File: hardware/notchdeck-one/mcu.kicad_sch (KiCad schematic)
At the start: 10 parts, among them J3 SWD, J4 TC2030_NL, U1 E73-2G4M08S1C

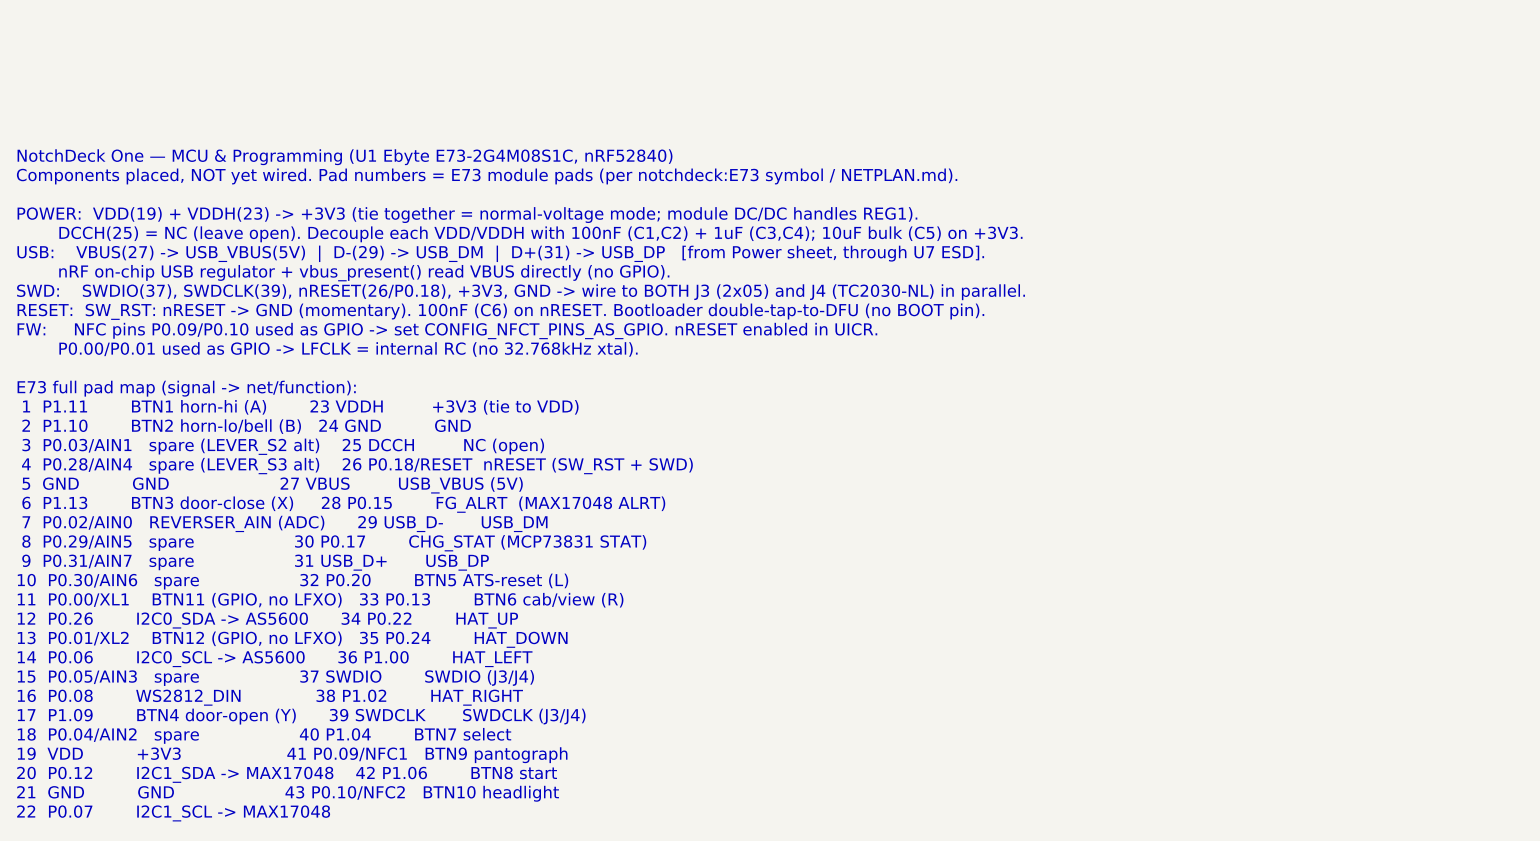
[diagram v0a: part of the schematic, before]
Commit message: Add schematic wiring notes support
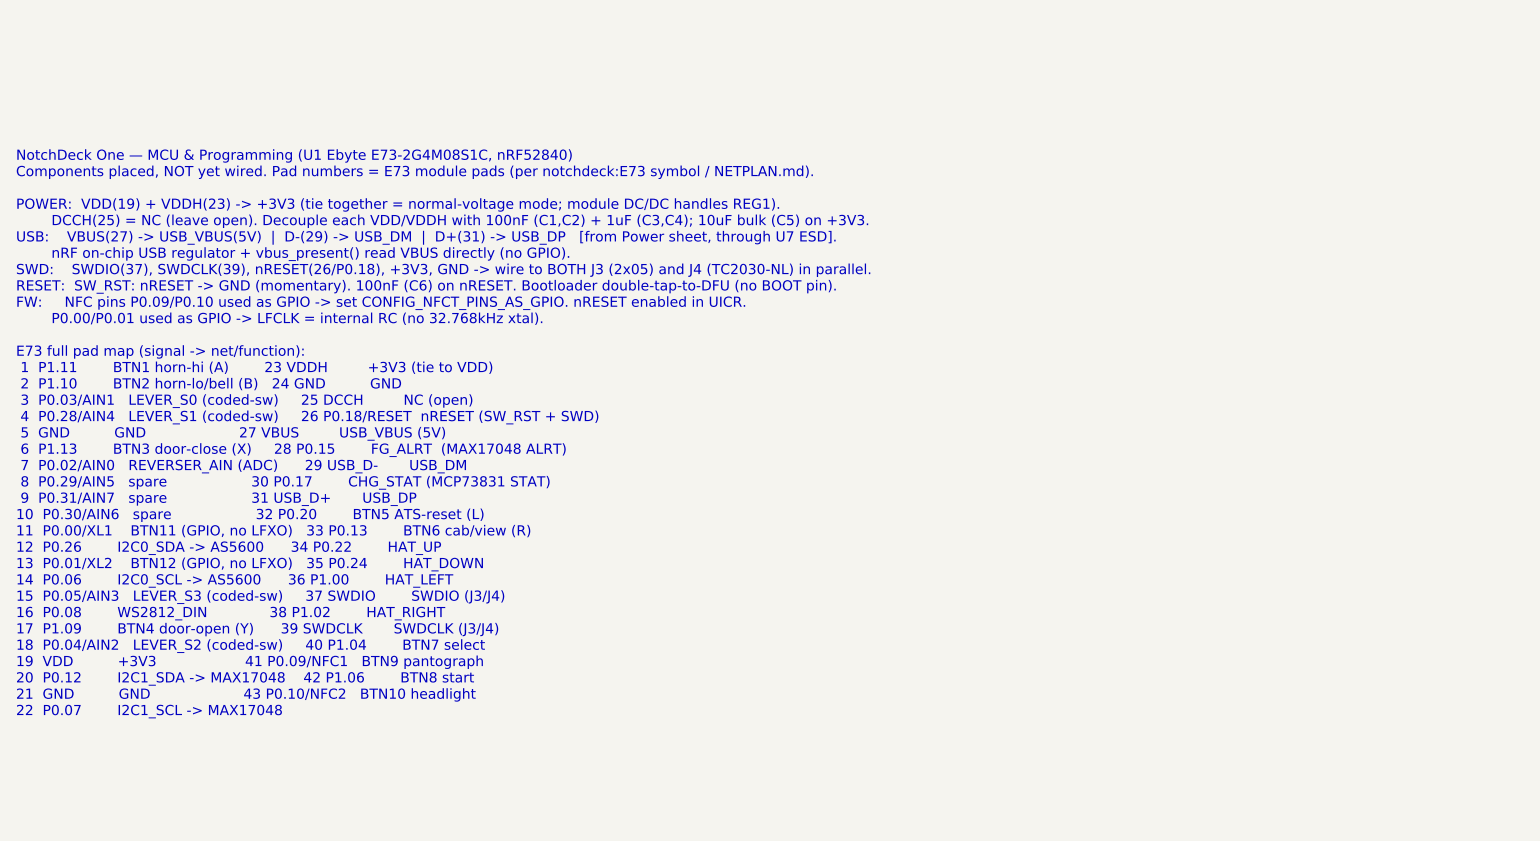
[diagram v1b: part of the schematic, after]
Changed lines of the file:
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@@
 		(instances
 			(project "notchdeck-one"
-				(path "/9b1c0f7a-1d2e-4a3b-8c5d-0e6f7a8b9c01/0d4eb303-8502-4a0e-80b0-eb5483675459"
+				(path "/9b1c0f7a-1d2e-4a3b-8c5d-0e6f7a8b9c01/69c9301a-7d1c-4dfc-8a82-adc2c5ab1b11"
 					(reference "U1")
 					(unit 1)
@@
 		(instances
 			(project "notchdeck-one"
-				(path "/9b1c0f7a-1d2e-4a3b-8c5d-0e6f7a8b9c01/0d4eb303-8502-4a0e-80b0-eb5483675459"
+				(path "/9b1c0f7a-1d2e-4a3b-8c5d-0e6f7a8b9c01/69c9301a-7d1c-4dfc-8a82-adc2c5ab1b11"
 					(reference "J3")
 					(unit 1)
@@
 		(instances
 			(project "notchdeck-one"
-				(path "/9b1c0f7a-1d2e-4a3b-8c5d-0e6f7a8b9c01/0d4eb303-8502-4a0e-80b0-eb5483675459"
+				(path "/9b1c0f7a-1d2e-4a3b-8c5d-0e6f7a8b9c01/69c9301a-7d1c-4dfc-8a82-adc2c5ab1b11"
 					(reference "J4")
 					(unit 1)
@@
 		(instances
 			(project "notchdeck-one"
-				(path "/9b1c0f7a-1d2e-4a3b-8c5d-0e6f7a8b9c01/0d4eb303-8502-4a0e-80b0-eb5483675459"
+				(path "/9b1c0f7a-1d2e-4a3b-8c5d-0e6f7a8b9c01/69c9301a-7d1c-4dfc-8a82-adc2c5ab1b11"
 					(reference "C1")
 					(unit 1)
@@
 		(instances
 			(project "notchdeck-one"
-				(path "/9b1c0f7a-1d2e-4a3b-8c5d-0e6f7a8b9c01/0d4eb303-8502-4a0e-80b0-eb5483675459"
+				(path "/9b1c0f7a-1d2e-4a3b-8c5d-0e6f7a8b9c01/69c9301a-7d1c-4dfc-8a82-adc2c5ab1b11"
 					(reference "C2")
 					(unit 1)
@@
 		(instances
 			(project "notchdeck-one"
-				(path "/9b1c0f7a-1d2e-4a3b-8c5d-0e6f7a8b9c01/0d4eb303-8502-4a0e-80b0-eb5483675459"
+				(path "/9b1c0f7a-1d2e-4a3b-8c5d-0e6f7a8b9c01/69c9301a-7d1c-4dfc-8a82-adc2c5ab1b11"
 					(reference "C3")
 					(unit 1)
@@
 		(instances
 			(project "notchdeck-one"
-				(path "/9b1c0f7a-1d2e-4a3b-8c5d-0e6f7a8b9c01/0d4eb303-8502-4a0e-80b0-eb5483675459"
+				(path "/9b1c0f7a-1d2e-4a3b-8c5d-0e6f7a8b9c01/69c9301a-7d1c-4dfc-8a82-adc2c5ab1b11"
 					(reference "C4")
 					(unit 1)
@@
 		(instances
 			(project "notchdeck-one"
-				(path "/9b1c0f7a-1d2e-4a3b-8c5d-0e6f7a8b9c01/0d4eb303-8502-4a0e-80b0-eb5483675459"
+				(path "/9b1c0f7a-1d2e-4a3b-8c5d-0e6f7a8b9c01/69c9301a-7d1c-4dfc-8a82-adc2c5ab1b11"
 					(reference "C5")
 					(unit 1)
@@
 		(instances
 			(project "notchdeck-one"
-				(path "/9b1c0f7a-1d2e-4a3b-8c5d-0e6f7a8b9c01/0d4eb303-8502-4a0e-80b0-eb5483675459"
+				(path "/9b1c0f7a-1d2e-4a3b-8c5d-0e6f7a8b9c01/69c9301a-7d1c-4dfc-8a82-adc2c5ab1b11"
 					(reference "C6")
 					(unit 1)
@@
 		(instances
 			(project "notchdeck-one"
-				(path "/9b1c0f7a-1d2e-4a3b-8c5d-0e6f7a8b9c01/0d4eb303-8502-4a0e-80b0-eb5483675459"
+				(path "/9b1c0f7a-1d2e-4a3b-8c5d-0e6f7a8b9c01/69c9301a-7d1c-4dfc-8a82-adc2c5ab1b11"
 					(reference "SW_RST")
 					(unit 1)
@@
 		)
 	)
-	(text "NotchDeck One — MCU & Programming (U1 Ebyte E73-2G4M08S1C, nRF52840)\nComponents placed, NOT yet wired. Pad numbers = E73 module pads (per notchdeck:E73 symbol / NETPLAN.md).\n\nPOWER:  VDD(19) + VDDH(23) -> +3V3 (tie together = normal-voltage mode; module DC/DC handles REG1).\n        DCCH(25) = NC (leave open). Decouple each VDD/VDDH with 100nF (C1,C2) + 1uF (C3,C4); 10uF bulk (C5) on +3V3.\nUSB:    VBUS(27) -> USB_VBUS(5V)  |  D-(29) -> USB_DM  |  D+(31) -> USB_DP   [from Power sheet, through U7 ESD].\n        nRF on-chip USB regulator + vbus_present() read VBUS directly (no GPIO).\nSWD:    SWDIO(37), SWDCLK(39), nRESET(26/P0.18), +3V3, GND -> wire to BOTH J3 (2x05) and J4 (TC2030-NL) in parallel.\nRESET:  SW_RST: nRESET -> GND (momentary). 100nF (C6) on nRESET. Bootloader double-tap-to-DFU (no BOOT pin).\nFW:     NFC pins P0.09/P0.10 used as GPIO -> set CONFIG_NFCT_PINS_AS_GPIO. nRESET enabled in UICR.\n        P0.00/P0.01 used as GPIO -> LFCLK = internal RC (no 32.768kHz xtal).\n\nE73 full pad map (signal -> net/function):\n 1  P1.11        BTN1 horn-hi (A)        23 VDDH         +3V3 (tie to VDD)\n 2  P1.10        BTN2 horn-lo/bell (B)   24 GND          GND\n 3  P0.03/AIN1   spare (LEVER_S2 alt)    25 DCCH         NC (open)\n 4  P0.28/AIN4   spare (LEVER_S3 alt)    26 P0.18/RESET  nRESET (SW_RST + SWD)\n 5  GND          GND                     27 VBUS         USB_VBUS (5V)\n 6  P1.13        BTN3 door-close (X)     28 P0.15        FG_ALRT  (MAX17048 ALRT)\n 7  P0.02/AIN0   REVERSER_AIN (ADC)      29 USB_D-       USB_DM\n 8  P0.29/AIN5   spare                   30 P0.17        CHG_STAT (MCP73831 STAT)\n 9  P0.31/AIN7   spare                   31 USB_D+       USB_DP\n10  P0.30/AIN6   spare                   32 P0.20        BTN5 ATS-reset (L)\n11  P0.00/XL1    BTN11 (GPIO, no LFXO)   33 P0.13        BTN6 cab/view (R)\n12  P0.26        I2C0_SDA -> AS5600      34 P0.22        HAT_UP\n13  P0.01/XL2    BTN12 (GPIO, no LFXO)   35 P0.24        HAT_DOWN\n14  P0.06        I2C0_SCL -> AS5600      36 P1.00        HAT_LEFT\n15  P0.05/AIN3   spare                   37 SWDIO        SWDIO (J3/J4)\n16  P0.08        WS2812_DIN              38 P1.02        HAT_RIGHT\n17  P1.09        BTN4 door-open (Y)      39 SWDCLK       SWDCLK (J3/J4)\n18  P0.04/AIN2   spare                   40 P1.04        BTN7 select\n19  VDD          +3V3                    41 P0.09/NFC1   BTN9 pantograph\n20  P0.12        I2C1_SDA -> MAX17048    42 P1.06        BTN8 start\n21  GND          GND                     43 P0.10/NFC2   BTN10 headlight\n22  P0.07        I2C1_SCL -> MAX17048"
+	(text "NotchDeck One — MCU & Programming (U1 Ebyte E73-2G4M08S1C, nRF52840)\nComponents placed, NOT yet wired. Pad numbers = E73 module pads (per notchdeck:E73 symbol / NETPLAN.md).\n\nPOWER:  VDD(19) + VDDH(23) -> +3V3 (tie together = normal-voltage mode; module DC/DC handles REG1).\n        DCCH(25) = NC (leave open). Decouple each VDD/VDDH with 100nF (C1,C2) + 1uF (C3,C4); 10uF bulk (C5) on +3V3.\nUSB:    VBUS(27) -> USB_VBUS(5V)  |  D-(29) -> USB_DM  |  D+(31) -> USB_DP   [from Power sheet, through U7 ESD].\n        nRF on-chip USB regulator + vbus_present() read VBUS directly (no GPIO).\nSWD:    SWDIO(37), SWDCLK(39), nRESET(26/P0.18), +3V3, GND -> wire to BOTH J3 (2x05) and J4 (TC2030-NL) in parallel.\nRESET:  SW_RST: nRESET -> GND (momentary). 100nF (C6) on nRESET. Bootloader double-tap-to-DFU (no BOOT pin).\nFW:     NFC pins P0.09/P0.10 used as GPIO -> set CONFIG_NFCT_PINS_AS_GPIO. nRESET enabled in UICR.\n        P0.00/P0.01 used as GPIO -> LFCLK = internal RC (no 32.768kHz xtal).\n\nE73 full pad map (signal -> net/function):\n 1  P1.11        BTN1 horn-hi (A)        23 VDDH         +3V3 (tie to VDD)\n 2  P1.10        BTN2 horn-lo/bell (B)   24 GND          GND\n 3  P0.03/AIN1   LEVER_S0 (coded-sw)     25 DCCH         NC (open)\n 4  P0.28/AIN4   LEVER_S1 (coded-sw)     26 P0.18/RESET  nRESET (SW_RST + SWD)\n 5  GND          GND                     27 VBUS         USB_VBUS (5V)\n 6  P1.13        BTN3 door-close (X)     28 P0.15        FG_ALRT  (MAX17048 ALRT)\n 7  P0.02/AIN0   REVERSER_AIN (ADC)      29 USB_D-       USB_DM\n 8  P0.29/AIN5   spare                   30 P0.17        CHG_STAT (MCP73831 STAT)\n 9  P0.31/AIN7   spare                   31 USB_D+       USB_DP\n10  P0.30/AIN6   spare                   32 P0.20        BTN5 ATS-reset (L)\n11  P0.00/XL1    BTN11 (GPIO, no LFXO)   33 P0.13        BTN6 cab/view (R)\n12  P0.26        I2C0_SDA -> AS5600      34 P0.22        HAT_UP\n13  P0.01/XL2    BTN12 (GPIO, no LFXO)   35 P0.24        HAT_DOWN\n14  P0.06        I2C0_SCL -> AS5600      36 P1.00        HAT_LEFT\n15  P0.05/AIN3   LEVER_S3 (coded-sw)     37 SWDIO        SWDIO (J3/J4)\n16  P0.08        WS2812_DIN              38 P1.02        HAT_RIGHT\n17  P1.09        BTN4 door-open (Y)      39 SWDCLK       SWDCLK (J3/J4)\n18  P0.04/AIN2   LEVER_S2 (coded-sw)     40 P1.04        BTN7 select\n19  VDD          +3V3                    41 P0.09/NFC1   BTN9 pantograph\n20  P0.12        I2C1_SDA -> MAX17048    42 P1.06        BTN8 start\n21  GND          GND                     43 P0.10/NFC2   BTN10 headlight\n22  P0.07        I2C1_SCL -> MAX17048"
 		(exclude_from_sim no)
 		(at 15.00 165.00 0)
-		(effects (font (size 1.5 1.5)) (justify left top))
+		(effects (font (face "Courier New") (size 1.27 1.27)) (justify left top))
 	)
 	(sheet_instances
